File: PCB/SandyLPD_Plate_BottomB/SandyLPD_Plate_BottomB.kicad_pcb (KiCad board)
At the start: 2 copper layers, 124.4 x 83 mm, 9 parts

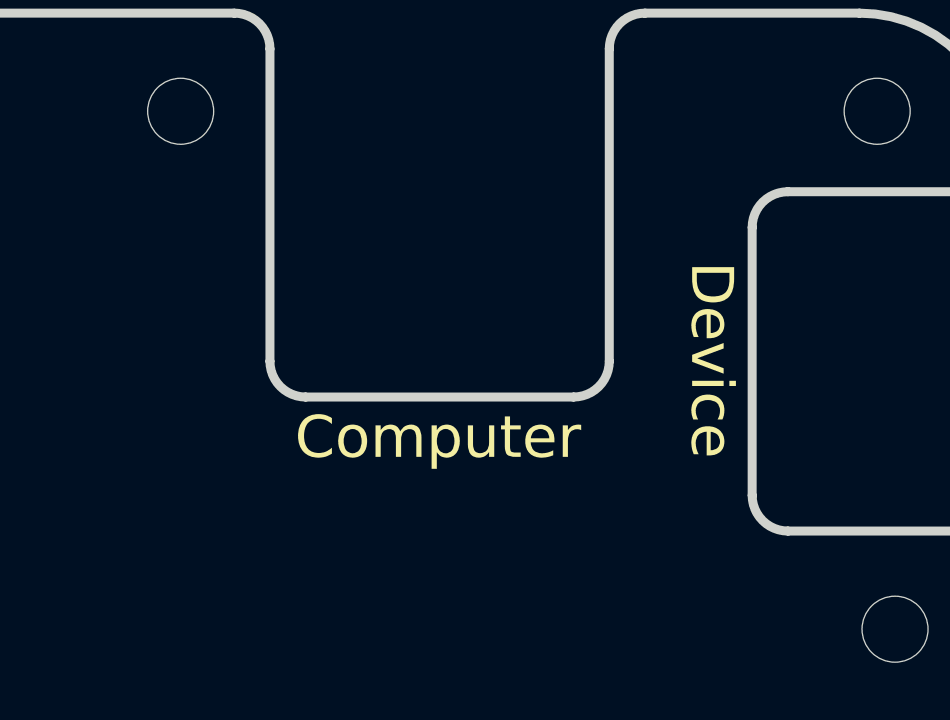
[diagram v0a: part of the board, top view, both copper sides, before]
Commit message: WIP　ボトムプレートへの記載を試し中
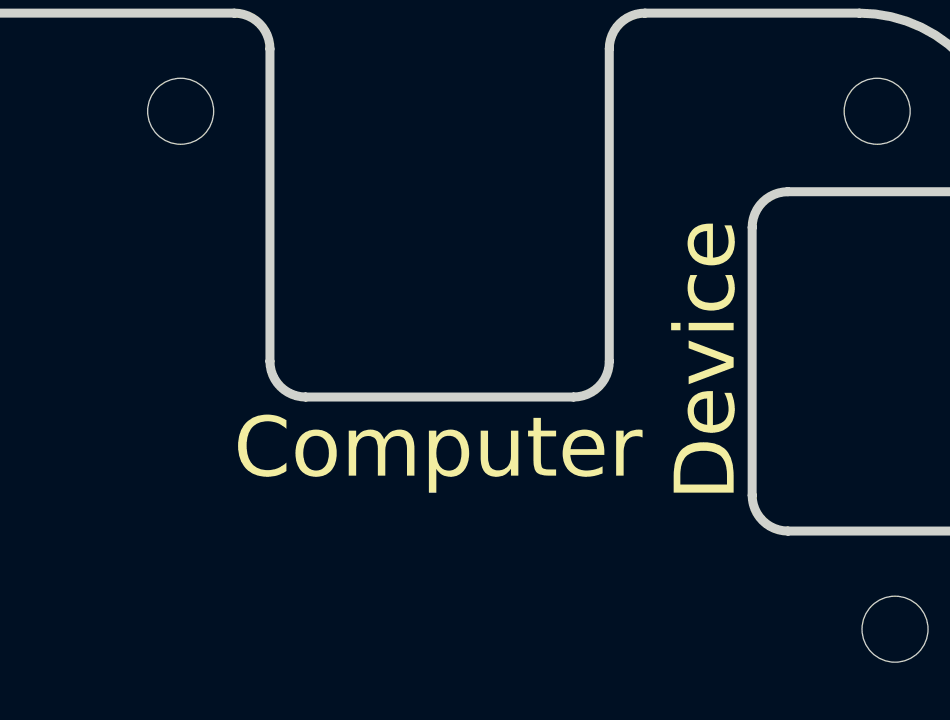
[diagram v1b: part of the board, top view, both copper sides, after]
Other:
- board text added: "⌨️"
